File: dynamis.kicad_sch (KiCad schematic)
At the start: 189 parts, among them J0 USB_C_Receptacle_USB2.0, SW00_00 SW_Push, SW00_01 SW_Push, SW00_02 SW_Push, SW00_03 SW_Push, SW00_04 SW_Push, SW00_05 SW_Push, SW00_06 SW_Push, SW01_00 SW_Push, SW01_01 SW_Push, SW01_02 SW_Push, SW01_03 SW_Push, SW01_04 SW_Push, SW01_05 SW_Push, SW01_06 SW_Push, SW02_01 SW_Push, SW02_02 SW_Push, SW02_03 SW_Push, SW02_04 SW_Push, SW02_05 SW_Push, SW02_06 SW_Push, SW03_00 SW_Push, SW03_02 SW_Push, SW03_03 SW_Push, SW03_04 SW_Push, SW03_05 SW_Push, SW03_06 SW_Push, SW04_00 SW_Push, SW04_01 SW_Push, SW04_02 SW_Push, SW04_03 SW_Push, SW04_05 SW_Push, SW04_06 SW_Push, SW05_01 SW_Push, SW05_02 SW_Push, SW05_03 SW_Push, SW05_04 SW_Push, SW05_05 SW_Push, SW05_06 SW_Push, SW06_00 SW_Push, SW06_01 SW_Push, SW06_02 SW_Push, SW06_03 SW_Push, SW06_04 SW_Push, SW06_05 SW_Push, SW06_06 SW_Push, SW07_01 SW_Push, SW07_02 SW_Push, SW07_03 SW_Push, SW07_04 SW_Push, SW07_05 SW_Push, SW07_06 SW_Push, SW08_00 SW_Push, SW08_02 SW_Push, SW08_03 SW_Push, SW08_04 SW_Push, SW08_05 SW_Push, SW08_06 SW_Push, SW09_00 SW_Push, SW09_01 SW_Push, SW09_02 SW_Push, SW09_03 SW_Push, SW09_04 SW_Push, SW09_05 SW_Push, SW09_06 SW_Push, U0 ATmega32U4-A, U1 PMW3360DM-T2QU, U2 TLV70019DDCR, U3 74LVC1T45GW,125, U4 74LVC1T45GW,125, U5 74LVC1T45GW,125, U6 74LVC1T45GW,125, U7 74LVC1T45GW,125, Y0 16Mhz

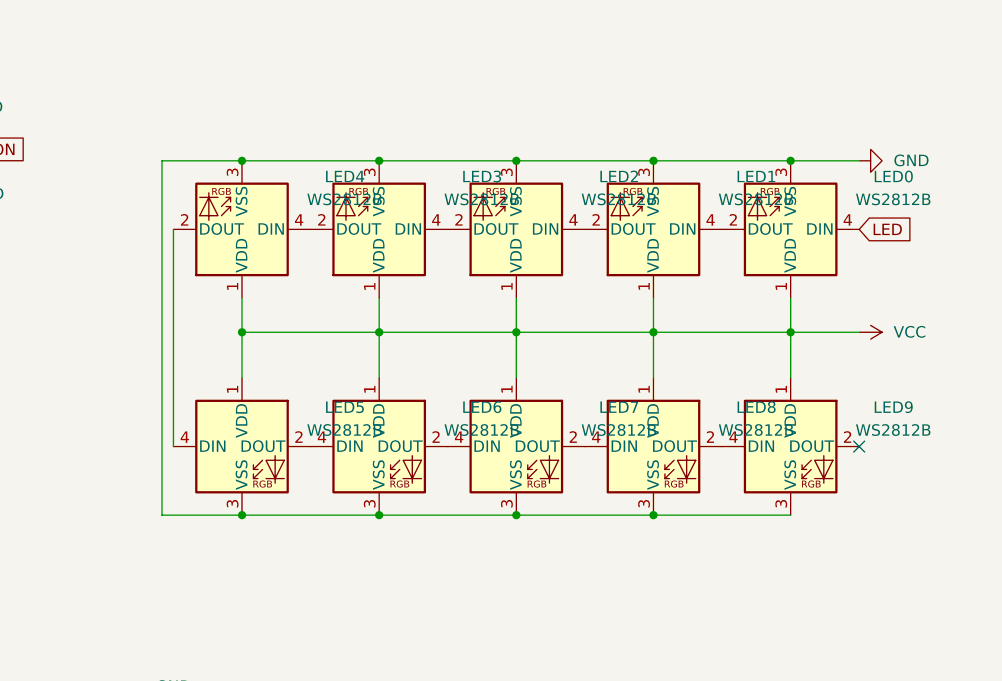
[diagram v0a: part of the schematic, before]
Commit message: initial as features (#1)
機能として完成した最初のコミット
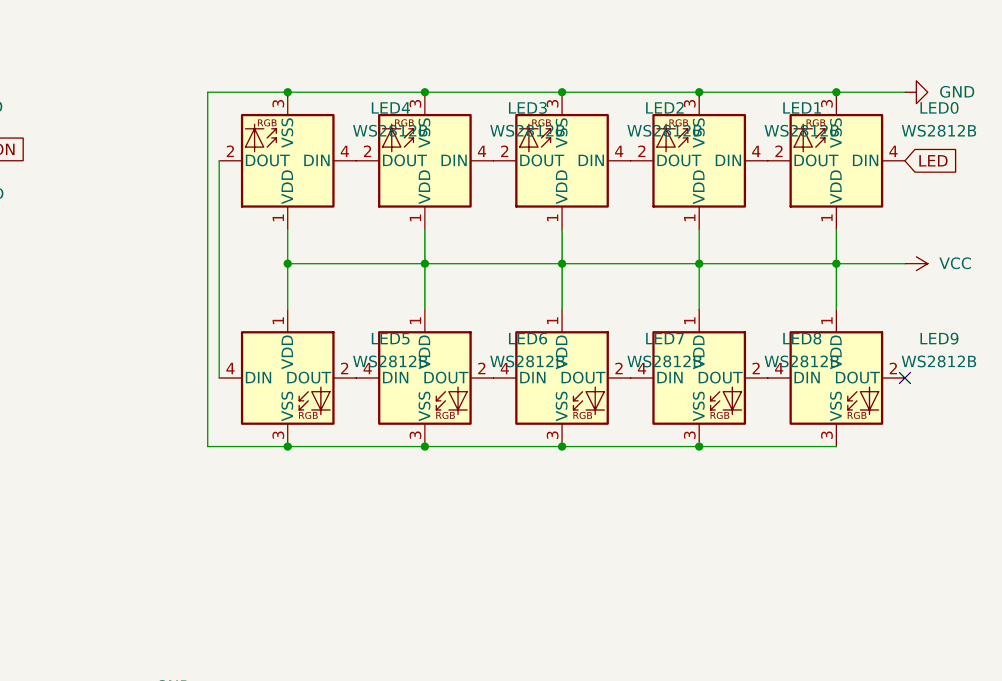
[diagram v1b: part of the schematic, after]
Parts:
- SW01_00: footprint MX_Only:MXOnly-1U-Hotswap -> MX_Only:MXOnly-1.5U-Hotswap
- SW03_00, SW04_00, SW04_01, SW04_02, SW04_06, SW09_05, SW09_06, SWSP_S04: footprint MX_Only:MXOnly-1U-Hotswap -> MX_Only:MXOnly-1.25U-Hotswap
- SW04_03: footprint MX_Only:MXOnly-1U-Hotswap -> MX_Only:MXOnly-2.25U-Hotswap-ReversedStabilizers
- SW04_05: footprint MX_Only:MXOnly-1U-Hotswap -> MX_Only:MXOnly-2.75U-Hotswap-ReversedStabilizers
- SWBS_L00: footprint MX_Only:MXOnly-1U-Hotswap -> MX_Only:MXOnly-2U-Hotswap
- SWCL_N00, SWRS_S01: footprint MX_Only:MXOnly-1U-Hotswap -> MX_Only:MXOnly-1.75U-Hotswap
- SWLS_L01: footprint MX_Only:MXOnly-1U-Hotswap -> MX_Only:MXOnly-2.25U-Hotswap
- SWRS_L01: footprint MX_Only:MXOnly-1U-Hotswap -> MX_Only:MXOnly-2.75U-Hotswap
- SWSP_L04: footprint MX_Only:MXOnly-1U-Hotswap -> MX_Only:MXOnly-6.25U-Hotswap
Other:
- moved on the sheet: LED0, LED1, LED2, LED3, LED6, LED7, LED8, LED9

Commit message: wip: switch layout
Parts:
- removed LED0, LED1, LED2, LED3, LED4, LED5, LED6, LED7, LED8, LED9: WS2812B, LED_SMD:LED_WS2812B_PLCC4_5.0x5.0mm_P3.2mm, symbol LED:WS2812B
- added LED00_00, LED00_01, LED00_02, LED00_03, LED00_04, LED00_05, LED00_06, LED01_00, LED01_01, LED01_02, LED01_03, LED01_04, LED01_05, LED01_06, LED02_00, LED02_01, LED02_02, LED02_03, LED02_04, LED02_05, LED02_06, LED03_00, LED03_01, LED03_02, LED03_03, LED03_04, LED03_05, LED03_06, LED04_00, LED04_01, LED04_02, LED04_03, LED04_04, LED04_05, LED04_06, LED05_00, LED05_01, LED05_02, LED05_03, LED05_04, LED05_05, LED05_06, LED06_00, LED06_01, LED06_02, LED06_03, LED06_04, LED06_05, LED06_06, LED07_00, LED07_01, LED07_02, LED07_03, LED07_04, LED07_05, LED07_06, LED08_00, LED08_01, LED08_02, LED08_03, LED08_04, LED08_05, LED08_06, LED09_00, LED09_01, LED09_02, LED09_03, LED09_04, LED09_05, LED09_06: SK6812MINI-E, SK6812MINI-E:SK6812MINIE, symbol SK6812MINI-E:SK6812MINI-E
- SWET_IS00: footprint MX_Only:MXOnly-1U-Hotswap -> MX_Only:MXOnly-2U-Hotswap-ReversedStabilizers
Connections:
- net GND: now also LED00_00.3 (GND), LED00_01.3 (GND), LED00_02.3 (GND), LED00_03.3 (GND), LED00_04.3 (GND), LED00_05.3 (GND), LED00_06.3 (GND), LED01_00.3 (GND), LED01_01.3 (GND), LED01_02.3 (GND), LED01_03.3 (GND), LED01_04.3 (GND), LED01_05.3 (GND), LED01_06.3 (GND), LED02_00.3 (GND), LED02_01.3 (GND), LED02_02.3 (GND), LED02_03.3 (GND), LED02_04.3 (GND), LED02_05.3 (GND), LED02_06.3 (GND), LED03_00.3 (GND), LED03_01.3 (GND), LED03_02.3 (GND), LED03_03.3 (GND), LED03_04.3 (GND), LED03_05.3 (GND), LED03_06.3 (GND), LED04_00.3 (GND), LED04_01.3 (GND), LED04_02.3 (GND), LED04_03.3 (GND), LED04_04.3 (GND), LED04_05.3 (GND), LED04_06.3 (GND), LED05_00.3 (GND), LED05_01.3 (GND), LED05_02.3 (GND), LED05_03.3 (GND), LED05_04.3 (GND), LED05_05.3 (GND), LED05_06.3 (GND), LED06_00.3 (GND), LED06_01.3 (GND), LED06_02.3 (GND), LED06_03.3 (GND), LED06_04.3 (GND), LED06_05.3 (GND), LED06_06.3 (GND), LED07_00.3 (GND), LED07_01.3 (GND), LED07_02.3 (GND), LED07_03.3 (GND), LED07_04.3 (GND), LED07_05.3 (GND), LED07_06.3 (GND), LED08_00.3 (GND), LED08_01.3 (GND), LED08_02.3 (GND), LED08_03.3 (GND), LED08_04.3 (GND), LED08_05.3 (GND), LED08_06.3 (GND), LED09_00.3 (GND), LED09_01.3 (GND), LED09_02.3 (GND), LED09_03.3 (GND), LED09_04.3 (GND), LED09_05.3 (GND), LED09_06.3 (GND)
- net LED: now also LED05_00.4 (DIN)
- net VCC: now also LED00_00.1 (VDD), LED00_01.1 (VDD), LED00_02.1 (VDD), LED00_03.1 (VDD), LED00_04.1 (VDD), LED00_05.1 (VDD), LED00_06.1 (VDD), LED01_00.1 (VDD), LED01_01.1 (VDD), LED01_02.1 (VDD), LED01_03.1 (VDD), LED01_04.1 (VDD), LED01_05.1 (VDD), LED01_06.1 (VDD), LED02_00.1 (VDD), LED02_01.1 (VDD), LED02_02.1 (VDD), LED02_03.1 (VDD), LED02_04.1 (VDD), LED02_05.1 (VDD), LED02_06.1 (VDD), LED03_00.1 (VDD), LED03_01.1 (VDD), LED03_02.1 (VDD), LED03_03.1 (VDD), LED03_04.1 (VDD), LED03_05.1 (VDD), LED03_06.1 (VDD), LED04_00.1 (VDD), LED04_01.1 (VDD), LED04_02.1 (VDD), LED04_03.1 (VDD), LED04_04.1 (VDD), LED04_05.1 (VDD), LED04_06.1 (VDD), LED05_00.1 (VDD), LED05_01.1 (VDD), LED05_02.1 (VDD), LED05_03.1 (VDD), LED05_04.1 (VDD), LED05_05.1 (VDD), LED05_06.1 (VDD), LED06_00.1 (VDD), LED06_01.1 (VDD), LED06_02.1 (VDD), LED06_03.1 (VDD), LED06_04.1 (VDD), LED06_05.1 (VDD), LED06_06.1 (VDD), LED07_00.1 (VDD), LED07_01.1 (VDD), LED07_02.1 (VDD), LED07_03.1 (VDD), LED07_04.1 (VDD), LED07_05.1 (VDD), LED07_06.1 (VDD), LED08_00.1 (VDD), LED08_01.1 (VDD), LED08_02.1 (VDD), LED08_03.1 (VDD), LED08_04.1 (VDD), LED08_05.1 (VDD), LED08_06.1 (VDD), LED09_00.1 (VDD), LED09_01.1 (VDD), LED09_02.1 (VDD), LED09_03.1 (VDD), LED09_04.1 (VDD), LED09_05.1 (VDD), LED09_06.1 (VDD)
- new net: LED04_04.4 (DIN), LED04_05.2 (DOUT)
- new net: LED03_05.2 (DOUT), LED04_05.4 (DIN)
- new net: LED00_06.4 (DIN), LED01_06.2 (DOUT)
- new net: LED01_06.4 (DIN), LED02_06.2 (DOUT)
- new net: LED09_02.2 (DOUT), LED09_03.4 (DIN)
- new net: LED08_02.2 (DOUT), LED09_02.4 (DIN)
- new net: LED00_02.4 (DIN), LED01_02.2 (DOUT)
- new net: LED01_02.4 (DIN), LED02_02.2 (DOUT)
- new net: LED05_06.2 (DOUT), LED06_06.4 (DIN)
- new net: LED05_05.2 (DOUT), LED05_06.4 (DIN)
- new net: LED07_05.4 (DIN), LED08_05.2 (DOUT)
- new net: LED08_05.4 (DIN), LED09_05.2 (DOUT)
- new net: LED00_01.2 (DOUT), LED01_01.4 (DIN)
- new net: LED00_01.4 (DIN), LED00_02.2 (DOUT)
- new net: LED09_00.2 (DOUT), LED09_01.4 (DIN)
- new net: LED08_00.2 (DOUT), LED09_00.4 (DIN)
- new net: LED05_04.2 (DOUT), LED06_04.4 (DIN)
- new net: LED05_03.2 (DOUT), LED05_04.4 (DIN)
- new net: LED08_01.4 (DIN), LED09_01.2 (DOUT)
- new net: LED02_06.4 (DIN), LED03_06.2 (DOUT)
- new net: LED03_06.4 (DIN), LED04_06.2 (DOUT)
- new net: LED01_01.2 (DOUT), LED02_01.4 (DIN)
- new net: LED07_02.2 (DOUT), LED08_02.4 (DIN)
- new net: LED01_03.2 (DOUT), LED02_03.4 (DIN)
- new net: LED00_03.2 (DOUT), LED01_03.4 (DIN)
- new net: LED07_00.2 (DOUT), LED08_00.4 (DIN)
- new net: LED00_05.4 (DIN), LED00_06.2 (DOUT)
- new net: LED06_00.2 (DOUT), LED07_00.4 (DIN)
- new net: LED05_01.2 (DOUT), LED05_02.4 (DIN)
- new net: LED05_01.4 (DIN), LED06_01.2 (DOUT)
- new net: LED06_01.4 (DIN), LED07_01.2 (DOUT)
- new net: LED07_01.4 (DIN), LED08_01.2 (DOUT)
- new net: LED06_04.2 (DOUT), LED07_04.4 (DIN)
- new net: LED03_00.4 (DIN), LED04_00.2 (DOUT)
- new net: LED04_00.4 (DIN), LED04_01.2 (DOUT)
- new net: LED08_04.2 (DOUT), LED09_04.4 (DIN)
- new net: LED07_04.2 (DOUT), LED08_04.4 (DIN)
- new net: LED00_03.4 (DIN), LED00_04.2 (DOUT)
- new net: LED00_04.4 (DIN), LED01_04.2 (DOUT)
- new net: LED09_04.2 (DOUT), LED09_05.4 (DIN)
- new net: LED03_02.4 (DIN), LED04_02.2 (DOUT)
- new net: LED04_02.4 (DIN), LED04_03.2 (DOUT)
- new net: LED06_02.2 (DOUT), LED07_02.4 (DIN)
- new net: LED01_05.2 (DOUT), LED02_05.4 (DIN)
- new net: LED00_05.2 (DOUT), LED01_05.4 (DIN)
- new net: LED02_02.4 (DIN), LED03_02.2 (DOUT)
- new net: LED06_03.4 (DIN), LED07_03.2 (DOUT)
- new net: LED07_03.4 (DIN), LED08_03.2 (DOUT)
- new net: LED00_00.4 (DIN), LED01_00.2 (DOUT)
- new net: LED01_04.4 (DIN), LED02_04.2 (DOUT)
- new net: LED02_00.4 (DIN), LED03_00.2 (DOUT)
- new net: LED07_06.2 (DOUT), LED08_06.4 (DIN)
- new net: LED06_06.2 (DOUT), LED07_06.4 (DIN)
- new net: LED03_04.4 (DIN), LED04_04.2 (DOUT)
- new net: LED04_06.4 (DIN), LED09_06.2 (DOUT)
- new net: LED08_03.4 (DIN), LED09_03.2 (DOUT)
- new net: LED05_00.2 (DOUT), LED06_00.4 (DIN)
- new net: LED02_01.2 (DOUT), LED03_01.4 (DIN)
- new net: LED05_03.4 (DIN), LED06_03.2 (DOUT)
- new net: LED08_06.2 (DOUT), LED09_06.4 (DIN)
- new net: LED06_05.4 (DIN), LED07_05.2 (DOUT)
- new net: LED02_05.2 (DOUT), LED03_05.4 (DIN)
- new net: LED03_03.2 (DOUT), LED04_03.4 (DIN)
- new net: LED02_04.4 (DIN), LED03_04.2 (DOUT)
- new net: LED05_02.2 (DOUT), LED06_02.4 (DIN)
- new net: LED05_05.4 (DIN), LED06_05.2 (DOUT)
- new net: LED03_01.2 (DOUT), LED04_01.4 (DIN)
- new net: LED01_00.4 (DIN), LED02_00.2 (DOUT)
- new net: LED02_03.2 (DOUT), LED03_03.4 (DIN)
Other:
- title: (none) -> dynamis
- moved on the sheet: C0, C1, C10, C2, C3, C4, C5, C6, C7, C8, C9, D00_00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

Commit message: wip
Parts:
- removed C5, C6: 1μF, Capacitor_SMD:C_1206_3216Metric, symbol Device:C
- removed JP0: SJ, Jumper:SolderJumper-2_P1.3mm_Open_Pad1.0x1.5mm, symbol Jumper:SolderJumper_2_Open
- removed LED00_00, LED00_01, LED00_02, LED00_03, LED00_04, LED00_05, LED00_06, LED01_00, LED01_01, LED01_02, LED01_03, LED01_04, LED01_05, LED01_06, LED02_00, LED02_01, LED02_02, LED02_03, LED02_04, LED02_05, LED02_06, LED03_00, LED03_01, LED03_02, LED03_03, LED03_04, LED03_05, LED03_06, LED04_00, LED04_01, LED04_02, LED04_03, LED04_04, LED04_05, LED04_06, LED05_01, LED05_02, LED05_03, LED05_04, LED05_05, LED05_06, LED06_01, LED06_02, LED06_03, LED06_04, LED06_05, LED06_06, LED07_01, LED07_02, LED07_03, LED07_04, LED07_05, LED07_06, LED08_01, LED08_02, LED08_03, LED08_04, LED08_05, LED08_06, LED09_01, LED09_02, LED09_03, LED09_04, LED09_05, LED09_06: SK6812MINI-E, SK6812MINI-E:SK6812MINIE, symbol SK6812MINI-E:SK6812MINI-E
- removed R7: 10k, Resistor_SMD:R_1206_3216Metric, symbol Device:R
- removed U0: ATmega32U4-A, Package_QFP:TQFP-44_10x10mm_P0.8mm, symbol MCU_Microchip_ATmega:ATmega32U4-A
- removed U2: TLV70019DDCR, TLV70019DDCR:Texas_Instruments-TLV70019DDCR-Level_A, symbol TLV70019DDCR:TLV70019DDCR
- removed U3, U4, U5, U6, U7: 74LVC1T45GW,125, 74LVC1T45GW:Nexperia-SOT363-11_2018-0-IPC_A, symbol 74LVC1T45GW:74LVC1T45GW,125
- added C10, C12, C16, C20: 10μF, Capacitor_SMD:C_1206_3216Metric, symbol Device:C
- added C11, C13, C15, C17, C19, C9: 0.1μF, Capacitor_SMD:C_1206_3216Metric, symbol Device:C
- added C14, C18: 1μF, Capacitor_SMD:C_1206_3216Metric, symbol Device:C
- added C21: 4.7μF, Capacitor_SMD:C_1206_3216Metric, symbol Device:C
- added ESDD0: ESD5Z5V0, Diode_SMD:D_SOD-523, symbol Diode:1.5KExxA
- added F0: SMD0805-050-16V, Fuse:Fuse_1206_3216Metric, symbol Device:Fuse
- added R10: 63.4K, Resistor_SMD:R_1206_3216Metric, symbol Device:R
- added R11: 52.3k, Resistor_SMD:R_1206_3216Metric, symbol Device:R
- added R12: 30.1k, Resistor_SMD:R_1206_3216Metric, symbol Device:R
- added R13: 1M, Resistor_SMD:R_1206_3216Metric, symbol Device:R
- added R5: 10k, Resistor_SMD:R_1206_3216Metric, symbol Device:R
- added R9: 37.4k, Resistor_SMD:R_1206_3216Metric, symbol Device:R
- added U0: ATmega32U4-M, Package_DFN_QFN:QFN-44-1EP_7x7mm_P0.5mm_EP5.2x5.2mm, symbol MCU_Microchip_ATmega:ATmega32U4-M
- added U2, U3: TPS73601DBV, Package_TO_SOT_SMD:SOT-23-5, symbol Regulator_Linear:TPS73601DBV
- added U4: TPD4E05U06DQAR, TPD4E05U06DQAR:USON-10_L2.5-W1.0-P0.50-BL, symbol random-keyboard-parts:TPD4E05U06DQAR
- added ZD_0, ZD_1, ZD_2: D_Zener, BZT52C3V3S:SOD-323_L1.6-W1.3-LS2.6-RD-1, symbol Device:D_Zener
- C0, C1: LCSC (none) -> C107174
- C2: LCSC (none) -> C1848
- C3: renamed from C7; LCSC (none) -> C24497
- C4: renamed from C8; LCSC (none) -> C24497
- C5: renamed from C9; LCSC (none) -> C24497
- C6: renamed from C10; LCSC (none) -> C13585
- C7: renamed from C3; LCSC (none) -> C29823
- C8: renamed from C4; LCSC (none) -> C24497
- D00_00, D00_01, D00_02, D00_03, D00_04, D00_05, D00_06, D01_00, D01_01, D01_02, D01_03, D01_04, D01_05, D01_06, D02_00, D02_01, D02_02, D02_03, D02_04, D02_05, D02_06, D03_00, D03_01, D03_02, D03_03, D03_04, D03_05, D03_06, D04_00, D04_01, D04_02, D04_03, D04_04, D04_05, D04_06, D05_00, D05_01, D05_02, D05_03, D05_04, D05_05, D05_06, D06_00, D06_01, D06_02, D06_03, D06_04, D06_05, D06_06, D07_00, D07_01, D07_02, D07_03, D07_04, D07_05, D07_06, D08_00, D08_01, D08_02, D08_03, D08_04, D08_05, D08_06, D09_00, D09_01, D09_02, D09_03, D09_04, D09_05, D09_06: LCSC (none) -> C81598
- J0: LCSC (none) -> C165948
- LED00: renamed from LED05_00; LCSC (none) -> C5149201
- LED01: renamed from LED06_00; LCSC (none) -> C5149201
- LED02: renamed from LED07_00; LCSC (none) -> C5149201
- LED03: renamed from LED08_00; LCSC (none) -> C5149201
- LED04: renamed from LED09_00; LCSC (none) -> C5149201
- R0, R1: LCSC (none) -> C17958
- R2, R8: LCSC (none) -> C17928
- R3, R4: LCSC (none) -> C964991
- R6: renamed from R5; LCSC (none) -> C17928
- R7: renamed from R6; LCSC (none) -> C286655
- RESET_SW0: LCSC (none) -> C318884
- SW00_00, SW00_01, SW00_02, SW00_03, SW00_04, SW00_05, SW00_06, SW01_00, SW01_01, SW01_02, SW01_03, SW01_04, SW01_05, SW01_06, SW02_01, SW02_02, SW02_03, SW02_04, SW02_05, SW02_06, SW03_00, SW03_02, SW03_03, SW03_04, SW03_05, SW03_06, SW04_00, SW04_01, SW04_02, SW04_03, SW04_05, SW04_06, SW05_01, SW05_02, SW05_03, SW05_04, SW05_05, SW05_06, SW06_00, SW06_01, SW06_02, SW06_03, SW06_04, SW06_05, SW06_06, SW07_01, SW07_02, SW07_03, SW07_04, SW07_05, SW07_06, SW08_00, SW08_02, SW08_03, SW08_04, SW08_05, SW08_06, SW09_00, SW09_01, SW09_02, SW09_03, SW09_04, SW09_05, SW09_06, SWBS_L00, SWBS_S00, SWCL_N00, SWCL_S00, SWET_AN00, SWET_IS00, SWLS_L01, SWLS_S01, SWRS_L01, SWRS_S01, SWSP_L04, SWSP_S04: LCSC (none) -> C5156480
- Y0: footprint Crystal:Crystal_SMD_SeikoEpson_FA238-4Pin_3.2x2.5mm -> X322516MLB4SI:OSC-SMD_4P-L3.2-W2.5-BL; LCSC (none) -> C13738
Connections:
- net D+: now also U4.4 (D2+), U4.5 (D2-), U4.6 (NC), U4.7 (NC)
- net D-: now also U4.1 (D1+), U4.10 (NC), U4.2 (D1-), U4.9 (NC)
- net GND: now also C7.2, C8.2, C10.2, C11.2, C12.2, C13.2, C14.2, C16.2, C17.2, C18.2, C20.2, C21.1, C9.2, ESDD0.2 (A2), R10.2, R12.2, R13.1, U0.15 (GND), U0.23 (GND), U0.35 (GND), U0.43 (GND), U0.45 (GND), U0.5 (UGND), U2.2 (GND), U3.2 (GND), U4.3 (GND), U4.8 (GND), ZD_0.2 (A), ZD_1.2 (A), ZD_2.2 (A); no longer C7.1, C8.1, J0.S1 (SHIELD)
- net LED: now also U0.1 (PE6)
- net MISO: now also R8.1, U0.11 (PB3)
- net MOSI: now also U0.10 (PB2), ZD_0.1 (K)
- net MOTION: now also U0.41 (PF0)
- net RESET: now also R5.2, U0.13 (~{RESET}); no longer R8.2
- net RE_A: now also U0.40 (PF1)
- net RE_B: now also U0.39 (PF4)
- net SCLK: now also U0.9 (PB1), ZD_1.1 (K)
- net VCC: now also ESDD0.1 (A1), F0.1; no longer C3.1, C4.1, C5.1, C6.1, LED00.1 (VDD), LED01.1 (VDD), LED02.1 (VDD), LED03.1 (VDD), LED04.1 (VDD), R8.1
- net col00: now also U0.18 (PD0)
- net col01: now also U0.19 (PD1)
- net col02: now also U0.37 (PF6)
- net col03: now also U0.36 (PF7)
- net col04: now also U0.22 (PD5)
- net col05: now also U0.12 (PB7)
- net col06: now also U0.38 (PF5)
- net row00: now also U0.27 (PD7)
- net row01: now also U0.26 (PD6)
- net row02: now also U0.25 (PD4)
- net row03: now also U0.21 (PD3)
- net row04: now also U0.20 (PD2)
- net row05: now also U0.28 (PB4)
- net row06: now also U0.29 (PB5)
- net row07: now also U0.30 (PB6)
- net row08: now also U0.31 (PC6)
- net row09: now also U0.32 (PC7)
- net at C2.1: now also U0.6 (UCAP)
- net at C0.2, Y0.3: now also U0.17 (XTAL1)
- net at R0.1: now also U0.4 (D+)
- net at C1.1, Y0.1: now also U0.16 (XTAL2)
- net at R2.2: now also U0.33 (~{HWB}/PE2)
- net at R1.1: now also U0.3 (D-)
- net SS renamed NCS
- net NCS: now also U0.8 (PB0), ZD_2.1 (K)
- net VDD renamed VDD_3_3v
- net VDD_3_3v: now also R8.2, C11.1, C12.1, C19.1, C20.1, R11.1, U3.5 (OUT); no longer R7.1, U1.4 (VDD)
- new net: C15.2, R10.1, R9.2, U2.4 (FB)
- new net: C19.2, R11.2, R12.1, U3.4 (FB)
- new net: C7.1, C8.1, U1.3 (VDDPIX)
- new net +5V: C13.1, C14.1, C17.1, C18.1, C3.1, C4.1, C5.1, C6.1, F0.2, LED00.1 (VDD), LED01.1 (VDD), LED02.1 (VDD), LED03.1 (VDD), LED04.1 (VDD), R5.1, U0.14 (VCC), U0.2 (UVCC), U0.24 (AVCC), U0.34 (VCC), U0.44 (AVCC), U0.7 (VBUS), U2.1 (IN), U2.3 (EN), U3.1 (IN), U3.3 (EN)
- new net GNDPWR: C21.2, J0.S1 (SHIELD), R13.2
- new net VDD_SS: C10.1, C15.1, C16.1, C9.1, R7.1, R9.1, U1.4 (VDD), U2.5 (OUT)
- no-connect marks 10 -> 9
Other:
- note added: "BADGE LED"
- note added: "Controller"
- note added: "ESD"
- note added: "Encoder"
- note added: "KEY MATRIX"
- note added: "PMW3360"
- moved on the sheet: C0, C1, C2, C3, C4, C5, C6, C7, C8, D00_00, D00_01, D00_02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

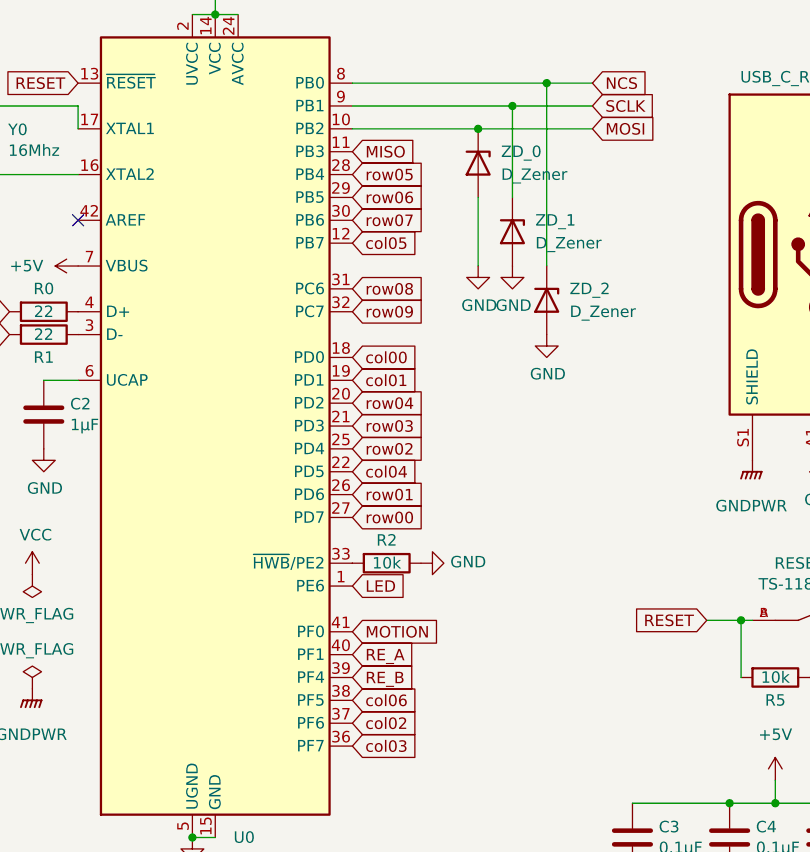
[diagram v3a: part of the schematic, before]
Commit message: wip
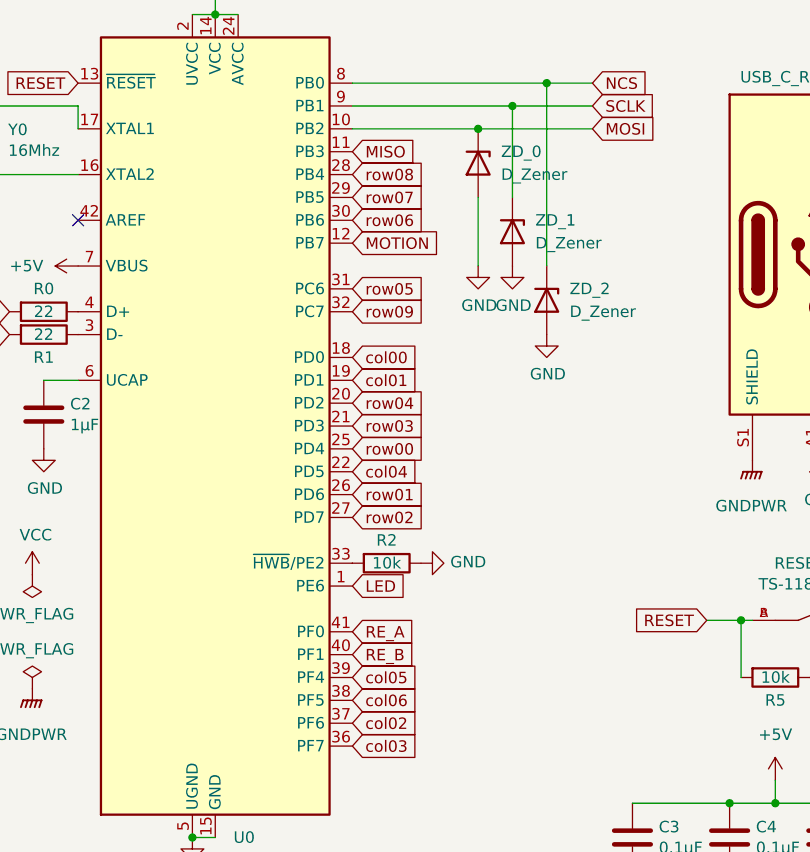
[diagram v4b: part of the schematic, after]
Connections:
- net MOTION: now also U0.12 (PB7); no longer U0.41 (PF0)
- net RE_A: now also U0.41 (PF0); no longer U0.40 (PF1)
- net RE_B: now also U0.40 (PF1); no longer U0.39 (PF4)
- net col05: now also U0.39 (PF4); no longer U0.12 (PB7)
- net row00: now also U0.25 (PD4); no longer U0.27 (PD7)
- net row02: now also U0.27 (PD7); no longer U0.25 (PD4)
- net row05: now also U0.31 (PC6); no longer U0.28 (PB4)
- net row06: now also U0.30 (PB6); no longer U0.29 (PB5)
- net row07: now also U0.29 (PB5); no longer U0.30 (PB6)
- net row08: now also U0.28 (PB4); no longer U0.31 (PC6)
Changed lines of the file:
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@@
     )
   )
-  (global_label "row08" (shape input) (at 88.9 77.47 0) (fields_autoplaced)
+  (global_label "row05" (shape input) (at 88.9 77.47 0) (fields_autoplaced)
     (effects (font (size 1.27 1.27)) (justify left))
     (property "Intersheet References" "${INTERSHEET_REFS}" (id 0) (at 96.9979 77.3906 0)
@@
     )
   )
-  (global_label "row00" (shape input) (at 88.9 102.87 0) (fields_autoplaced)
+  (global_label "row02" (shape input) (at 88.9 102.87 0) (fields_autoplaced)
     (effects (font (size 1.27 1.27)) (justify left))
     (property "Intersheet References" "${INTERSHEET_REFS}" (id 0) (at 96.9979 102.7906 0)
@@
     )
   )
-  (global_label "row05" (shape input) (at 88.9 64.77 0) (fields_autoplaced)
+  (global_label "row08" (shape input) (at 88.9 64.77 0) (fields_autoplaced)
     (effects (font (size 1.27 1.27)) (justify left))
     (property "Intersheet References" "${INTERSHEET_REFS}" (id 0) (at 96.9979 64.6906 0)
@@
     )
   )
-  (global_label "row06" (shape input) (at 88.9 67.31 0) (fields_autoplaced)
-    (effects (font (size 1.27 1.27)) (justify left))
-    (property "Intersheet References" "${INTERSHEET_REFS}" (id 0) (at 96.909 67.2306 0)
-      (effects (font (size 1.27 1.27)) (justify left) hide)
-    )
-  )
-  (global_label "row02" (shape input) (at 88.9 95.25 0) (fields_autoplaced)
+  (global_label "row07" (shape input) (at 88.9 67.31 0) (fields_autoplaced)
+    (effects (font (size 1.27 1.27)) (justify left))
+    (property "Intersheet References" "${INTERSHEET_REFS}" (id 0) (at 96.9979 67.2306 0)
+      (effects (font (size 1.27 1.27)) (justify left) hide)
+    )
+  )
+  (global_label "row00" (shape input) (at 88.9 95.25 0) (fields_autoplaced)
     (effects (font (size 1.27 1.27)) (justify left))
     (property "Intersheet References" "${INTERSHEET_REFS}" (id 0) (at 96.9979 95.1706 0)
@@
     )
   )
-  (global_label "col05" (shape input) (at 88.9 72.39 0) (fields_autoplaced)
-    (effects (font (size 1.27 1.27)) (justify left))
-    (property "Intersheet References" "${INTERSHEET_REFS}" (id 0) (at 96.635 72.3106 0)
+  (global_label "MOTION" (shape input) (at 88.9 72.39 0) (fields_autoplaced)
+    (effects (font (size 1.27 1.27)) (justify left))
+    (property "Intersheet References" "${INTERSHEET_REFS}" (id 0) (at 98.3283 72.3106 0)
       (effects (font (size 1.27 1.27)) (justify left) hide)
     )
@@
     )
   )
-  (global_label "row07" (shape input) (at 88.9 69.85 0) (fields_autoplaced)
+  (global_label "row06" (shape input) (at 88.9 69.85 0) (fields_autoplaced)
     (effects (font (size 1.27 1.27)) (justify left))
     (property "Intersheet References" "${INTERSHEET_REFS}" (id 0) (at 96.9979 69.7706 0)
@@
     )
   )
-  (global_label "RE_A" (shape input) (at 88.9 118.11 0) (fields_autoplaced)
-    (effects (font (size 1.27 1.27)) (justify left))
-    (property "Intersheet References" "${INTERSHEET_REFS}" (id 0) (at 95.7883 118.0306 0)
+  (global_label "RE_B" (shape input) (at 88.9 118.11 0) (fields_autoplaced)
+    (effects (font (size 1.27 1.27)) (justify left))
+    (property "Intersheet References" "${INTERSHEET_REFS}" (id 0) (at 95.9698 118.0306 0)
       (effects (font (size 1.27 1.27)) (justify left) hide)
     )
@@
     )
   )
-  (global_label "RE_B" (shape input) (at 88.9 120.65 0) (fields_autoplaced)
-    (effects (font (size 1.27 1.27)) (justify left))
-    (property "Intersheet References" "${INTERSHEET_REFS}" (id 0) (at 95.9698 120.5706 0)
+  (global_label "col05" (shape input) (at 88.9 120.65 0) (fields_autoplaced)
+    (effects (font (size 1.27 1.27)) (justify left))
+    (property "Intersheet References" "${INTERSHEET_REFS}" (id 0) (at 96.635 120.5706 0)
       (effects (font (size 1.27 1.27)) (justify left) hide)
     )
@@
     )
   )
-  (global_label "MOTION" (shape input) (at 88.9 115.57 0) (fields_autoplaced)
-    (effects (font (size 1.27 1.27)) (justify left))
-    (property "Intersheet References" "${INTERSHEET_REFS}" (id 0) (at 98.3283 115.4906 0)
-      (effects (font (size 1.27 1.27)) (justify left) hide)
-    )
+  (global_label "RE_A" (shape input) (at 88.9 115.57 0) (fields_autoplaced)
+    (effects (font (size 1.27 1.27)) (justify left))
+    (property "Intersheet References" "${INTERSHEET_REFS}" (id 0) (at 95.7883 115.4906 0)
+      (effects (font (size 1.27 1.27)) (justify left) hide)
+    )
